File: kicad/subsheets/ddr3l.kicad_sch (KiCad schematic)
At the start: 29 parts, among them U6 MT41K256M16TW-107:P

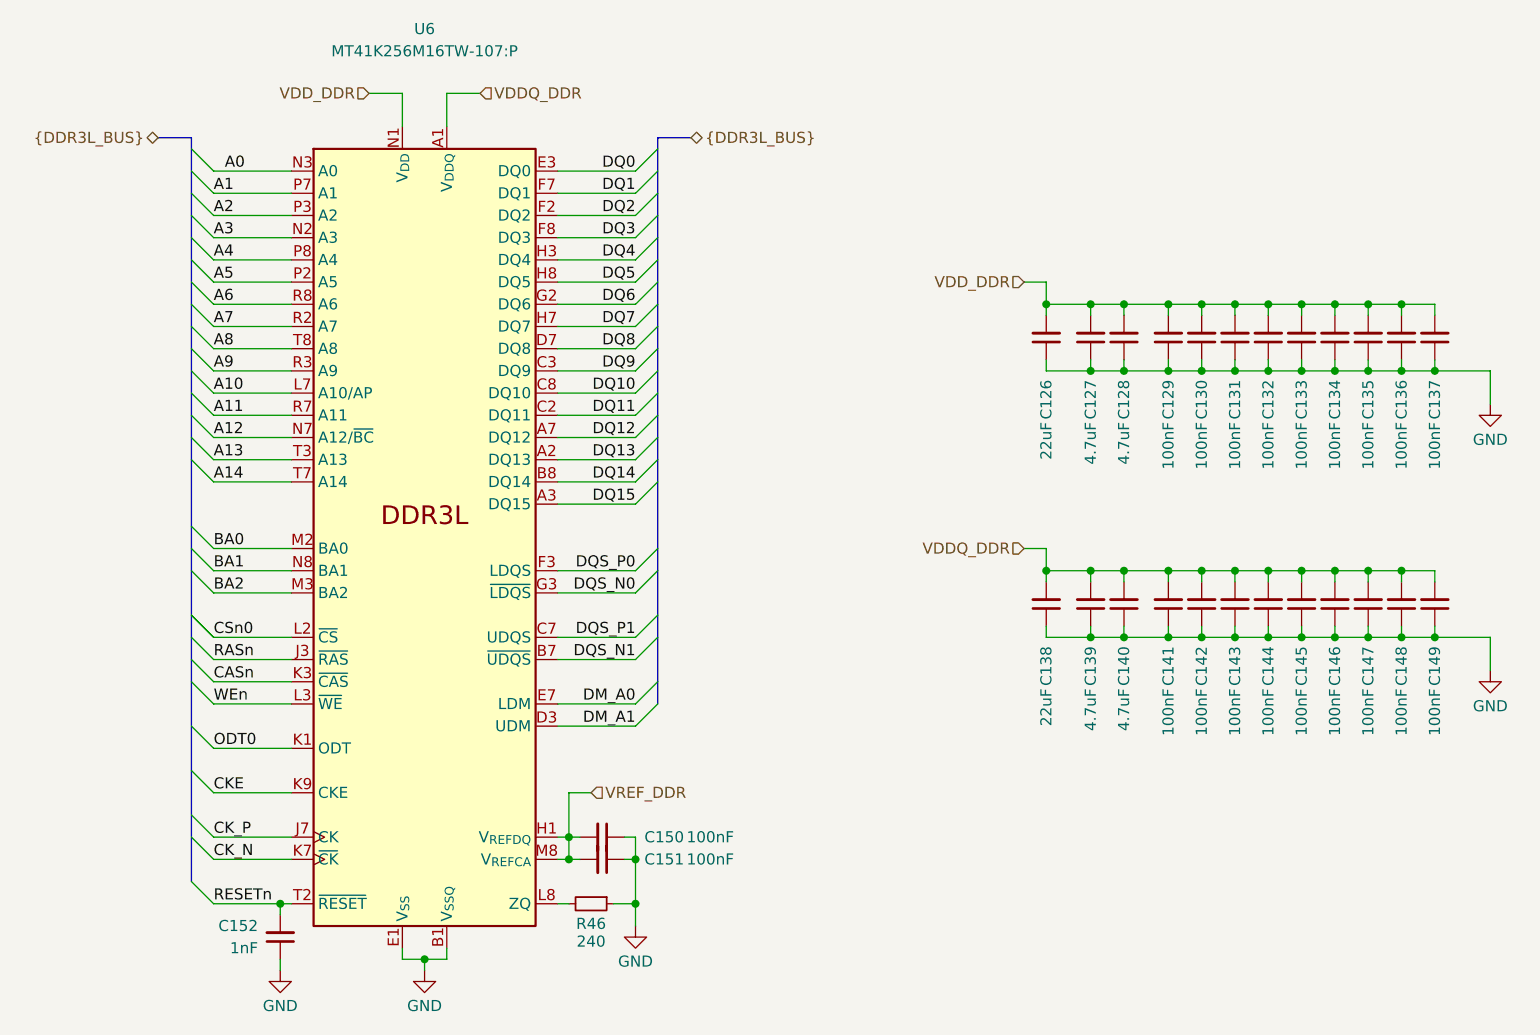
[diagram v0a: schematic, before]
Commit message: Annotations
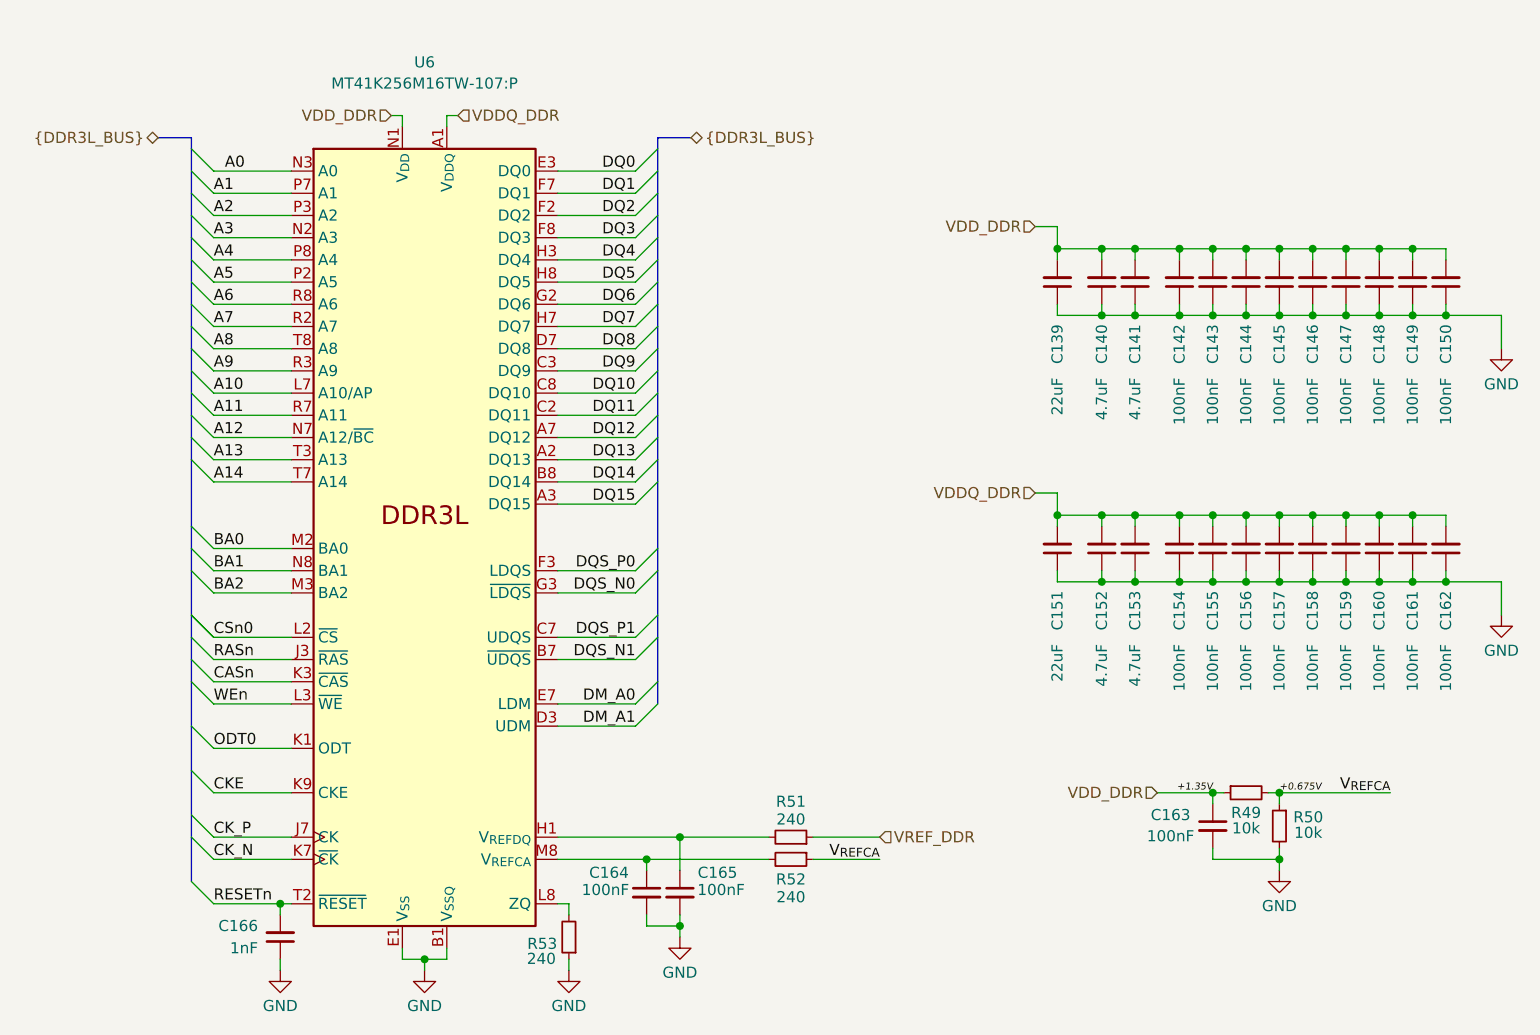
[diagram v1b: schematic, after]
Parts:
- removed C150, C151: 100nF, symbol Device:C_Small
- added C163, C164, C165: 100nF, symbol Device:C_Small
- added R49, R50: 10k, symbol Device:R_Small
- added R51, R52: 240, symbol Device:R_Small
- renumbered C126 to C139, C127 to C140, C128 to C141, C129 to C142, C130 to C143, C131 to C144, C132 to C145, C133 to C146, C134 to C147, C135 to C148, C136 to C149, C137 to C150, C138 to C151, C139 to C152, C140 to C153, C141 to C154, C142 to C155, C143 to C156, C144 to C157, C145 to C158, C146 to C159, C147 to C160, C148 to C161, C149 to C162, C152 to C166, R46 to R53
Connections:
- net GND: now also C163.2, C164.2, C165.2, R50.2
- net VDD_DDR: now also C163.1, R49.1
- net VREF_DDR: now also R51.1; no longer U6.H1 (V_{REFDQ}), U6.M8 (V_{REFCA})
- new net: C165.1, R51.2, U6.H1 (V_{REFDQ})
- new net: C164.1, R52.2, U6.M8 (V_{REFCA})
- new net +0.675V: R49.2, R50.1, R52.1
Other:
- moved on the sheet: C139, C140, C141, C142, C143, C144, C145, C146, C147, C148, C149, C150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
